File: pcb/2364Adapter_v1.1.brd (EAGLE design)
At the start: 35.6 x 21.6 mm, 10 parts, among them IC1 2364, IC2 EPROM

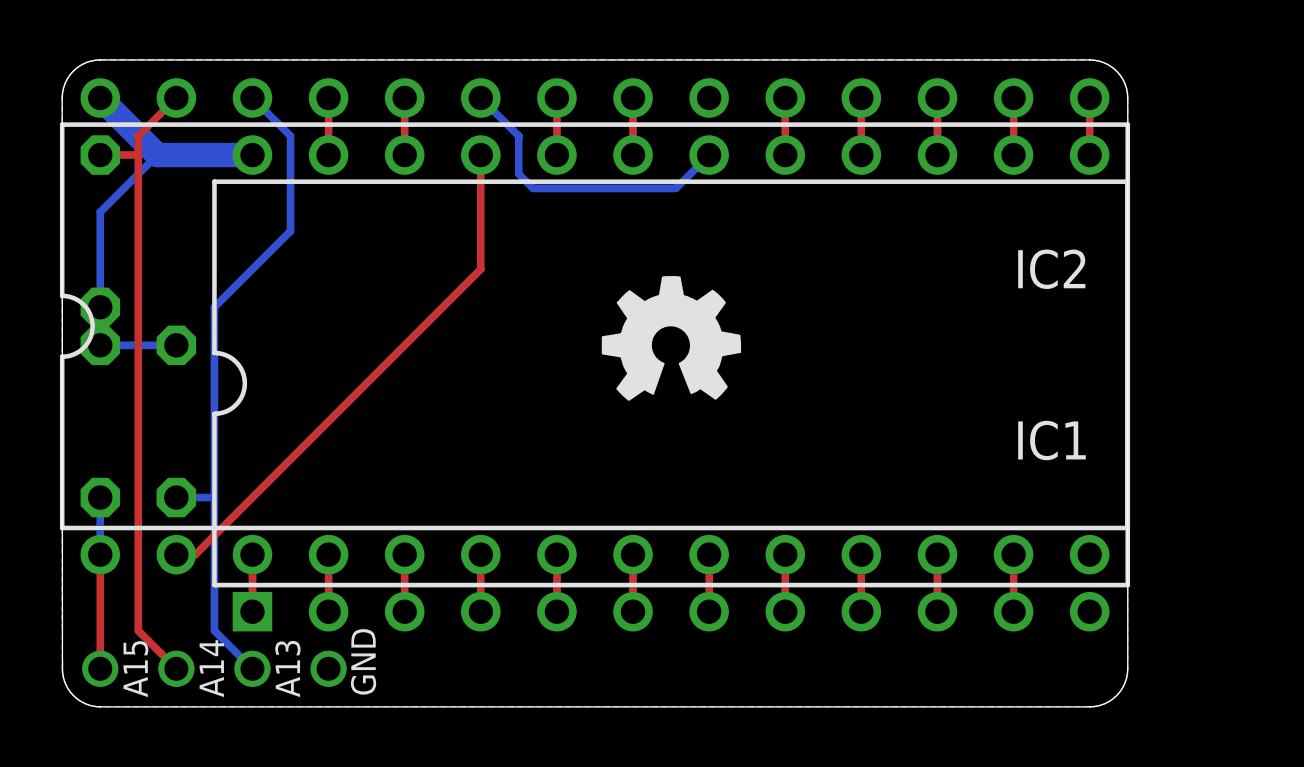
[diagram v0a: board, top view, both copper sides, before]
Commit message: Added media
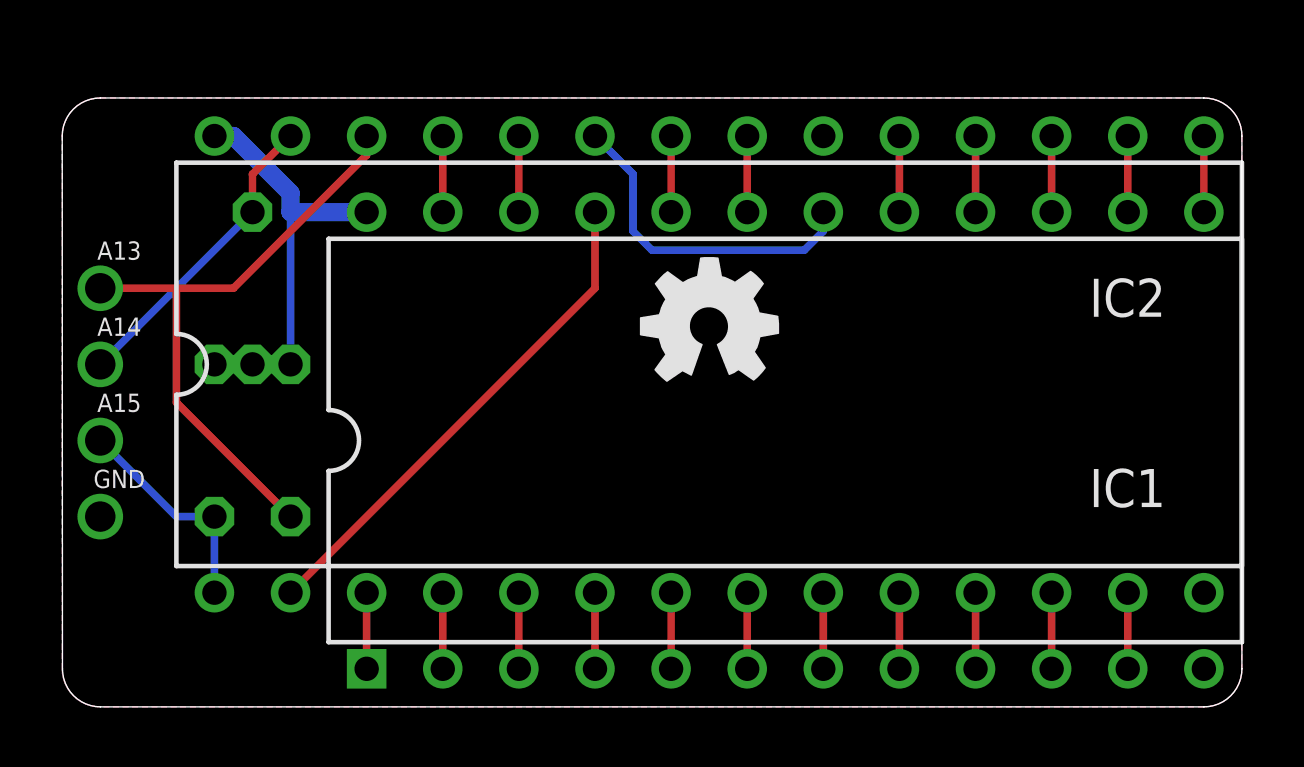
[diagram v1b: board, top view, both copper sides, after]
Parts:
- removed A13, A14, A15, GND: TPTP12R, testpad:TP12R
- added X1: (no value), con-lstb-rp:MA04-1
- moved R2 5.43 mm to (6.35, 14.0)
- moved IC1 4.26 mm to (24.1, 8.89)
- moved IC2 4.02 mm to (21.6, 11.4)
- moved R1 3.86 mm to (7.62, 8.89)
- moved R3 3.86 mm to (5.08, 8.89)
- moved GOLD_ORB_SM1 1.42 mm to (21.6, 12.7)
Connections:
- net A13: now also X1.4; no longer A13.TP
- net A14: now also X1.3; no longer A14.TP
- net A15: now also X1.2; no longer A15.TP
- net GND: now also X1.1; no longer GND.TP
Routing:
- net A14: track 21.4 -> 10.3 mm, vias 1 -> 0
- net A13: track 22.4 -> 20.6 mm, vias 1 -> 0
- net A15: track 5.71 -> 7.40 mm, vias 1 -> 0
- net A11: track 10.1 -> 11.2 mm
- net A12: track 17.9 -> 16.9 mm
- net D2: track 1.91 -> 2.54 mm
- net D1: track 1.91 -> 2.54 mm
- net D0: track 1.91 -> 2.54 mm
- net A7: track 1.91 -> 2.54 mm
- net A6: track 1.91 -> 2.54 mm
- net A5: track 1.91 -> 2.54 mm
- net A4: track 1.91 -> 2.54 mm
- net A3: track 1.91 -> 2.54 mm
- net A2: track 1.91 -> 2.54 mm
- net A1: track 1.91 -> 2.54 mm
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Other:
- board size 35.6 x 21.6 mm -> 39.4 x 20.3 mm
- board text added: "A13"
- board text added: "A14"
- board text added: "A15"
- board text added: "GND"
